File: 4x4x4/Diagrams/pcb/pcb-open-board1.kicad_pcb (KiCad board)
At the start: 2 copper layers, 87.6 x 110.5 mm, 77 parts, among them J1 DB128V-5_0-4P, J10 DB128V-5_0-4P, J11 DB128V-5_0-4P, J12 DB128V-5_0-4P, J13 DB128V-5_0-4P, J14 DB128V-5_0-4P, J2 DB128V-5_0-6P, J3 DB128V-5_0-4P, J4 DB128V-5_0-4P, J5 DB128V-5_0-4P, J6 DB128V-5_0-4P, J7 DB128V-5_0-4P, J8 DB128V-5_0-4P, J9 DB128V-5_0-4P, Q1 2N2222, Q2 2N2222, Q3 2N2222, Q4 2N2222, U1 74HC595D,118, U2 74HC595D,118, U3 74HC595D,118, U4 74HC595D,118, U5 74HC595D,118, U6 locked, U7 74HC595D,118

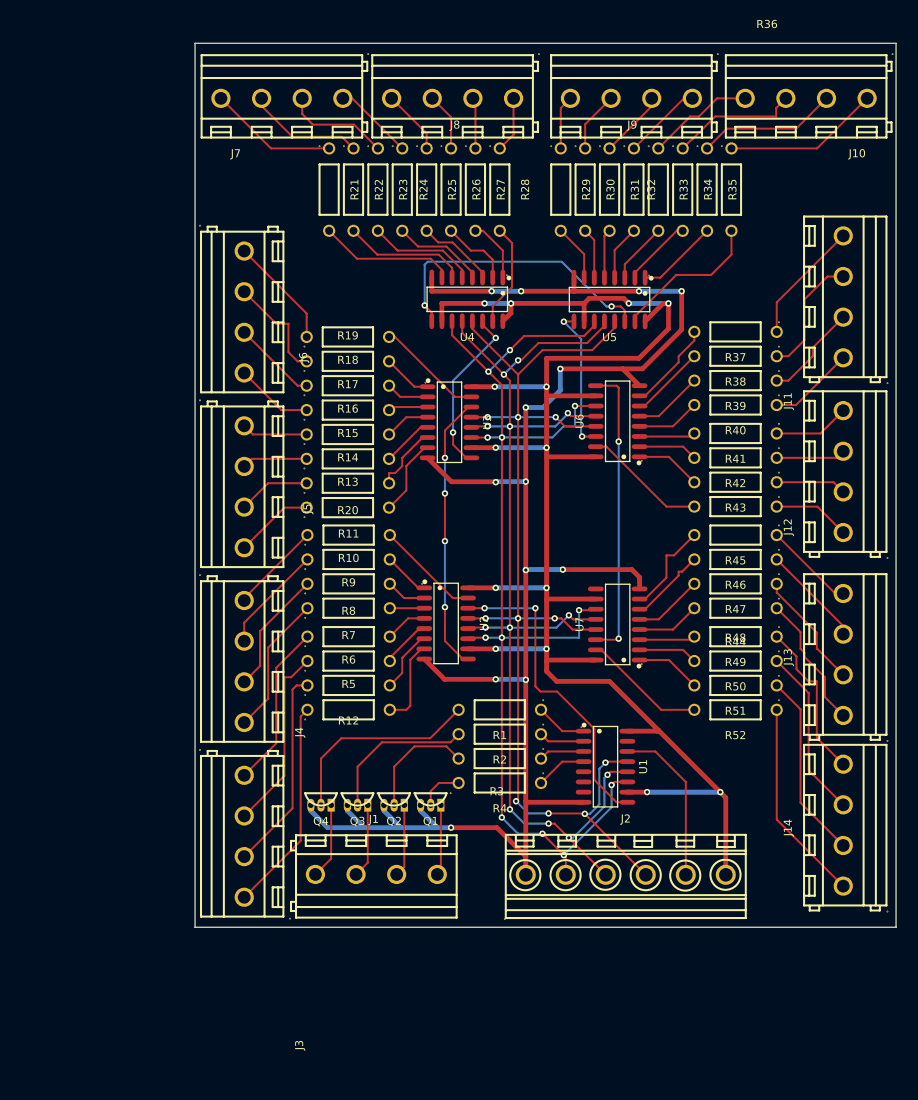
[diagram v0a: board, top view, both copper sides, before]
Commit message: create new board
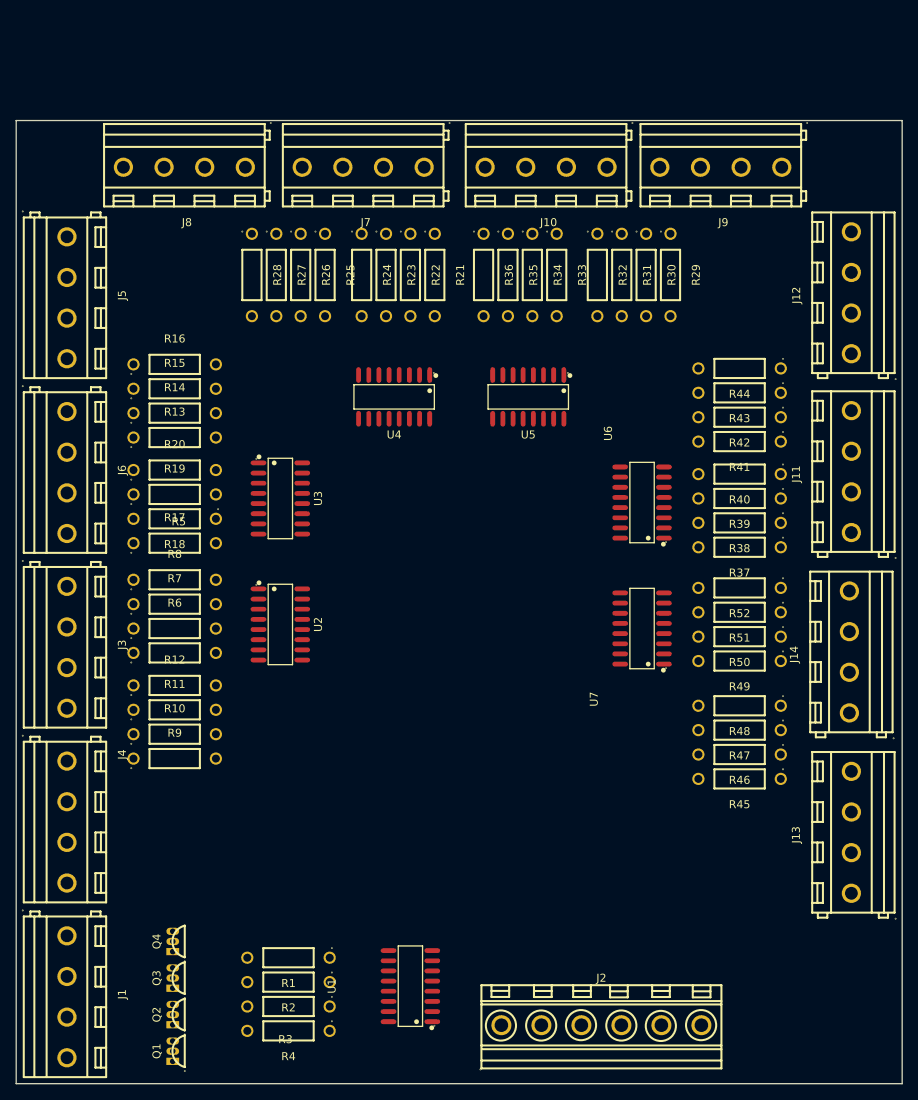
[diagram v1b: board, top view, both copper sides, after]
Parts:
- U6: value locked -> 74HC595D,118
- moved Q1 44.5 mm to (51.9, 175.4), turned to 90 degrees
- moved J1 41.3 mm to (37.6, 168.2), turned to -90 degrees
- moved R1 40.7 mm to (65.6, 163.7)
- moved R2 40.7 mm to (65.6, 166.7)
- moved R3 40.7 mm to (65.6, 169.8)
- moved R4 40.7 mm to (65.6, 172.8)
- moved Q2 38.1 mm to (51.9, 170.8), turned to 90 degrees
- moved U1 36.7 mm to (80.8, 167.2), turned to 90 degrees
- moved J8 34.6 mm to (52.9, 64.6)
- moved J10 33.6 mm to (98.1, 64.6)
- moved R28 32.8 mm to (61.0, 78.3)
- moved R36 32.8 mm to (90.0, 78.3)
- moved J3 32.4 mm to (37.6, 124.6)
- moved J5 32.4 mm to (37.6, 80.9)
- moved Q3 31.6 mm to (51.9, 166.2), turned to 90 degrees
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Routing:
- net GND: track 217.6 -> 0.00 mm, vias 13 -> 0
- net Net-(J2-Pad6): track 216.3 -> 0.00 mm, vias 14 -> 0
- net Net-(J2-Pad2): track 144.6 -> 0.00 mm, vias 12 -> 0
- net Net-(J2-Pad3): track 140.7 -> 0.00 mm, vias 12 -> 0
- net Net-(J2-Pad4): track 140.0 -> 0.00 mm, vias 10 -> 0
- net Net-(U1-Pad9): track 39.4 -> 0.00 mm, vias 2 -> 0
- net Net-(U6-Pad9): track 37.3 -> 0.00 mm, vias 2 -> 0
- net Net-(U4-Pad9): track 36.5 -> 0.00 mm, vias 2 -> 0
- net Net-(U2-Pad9): track 34.6 -> 0.00 mm, vias 4 -> 0
- net Net-(J3-Pad4): track 26.7 -> 0.00 mm
- net Net-(Q4-Pad2): track 25.6 -> 0.00 mm
- net Net-(J14-Pad1): track 25.5 -> 0.00 mm
- net Net-(J3-Pad3): track 25.5 -> 0.00 mm
- net Net-(J14-Pad2): track 23.5 -> 0.00 mm
- net Net-(J3-Pad2): track 23.1 -> 0.00 mm
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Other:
- board size 87.6 x 110.5 mm -> 110.7 x 120.4 mm
